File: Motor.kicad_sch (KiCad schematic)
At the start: 5 parts, among them U8 DRV8833PW

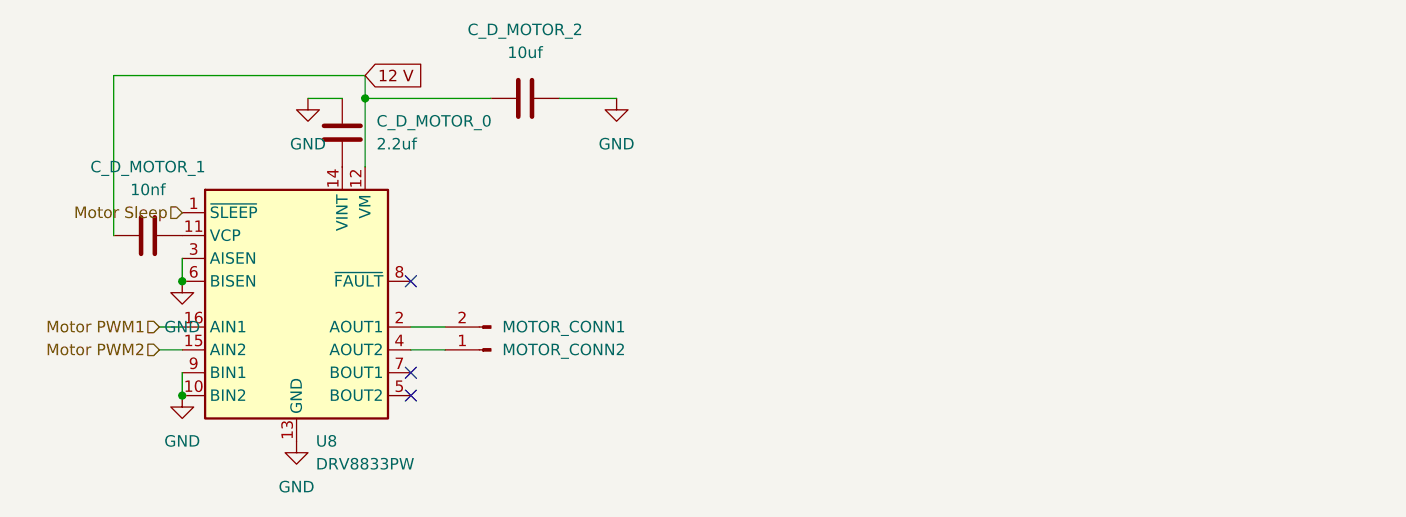
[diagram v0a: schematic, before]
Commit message: footprints
footprints
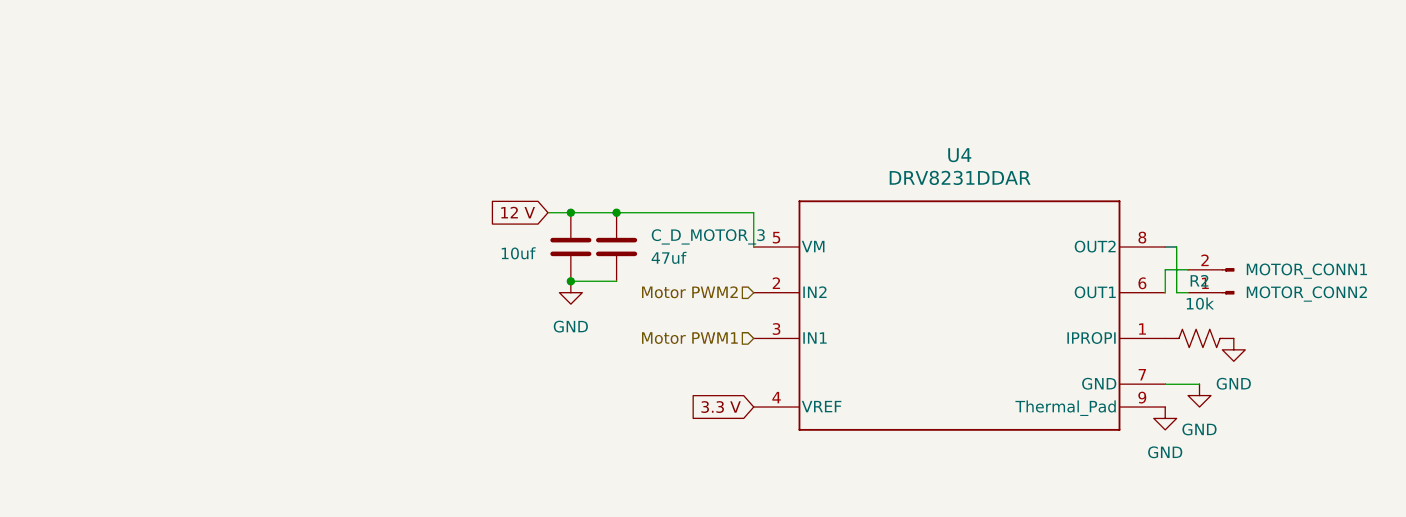
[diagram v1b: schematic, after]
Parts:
- removed C_D_MOTOR_0: 2.2uf, symbol Device:C
- removed C_D_MOTOR_1: 10nf, symbol Device:C
- removed U8: DRV8833PW, Package_SO:TSSOP-16_4.4x5mm_P0.65mm, symbol Driver_Motor:DRV8833PW
- added C_D_MOTOR_3: 47uf, Capacitor_SMD:C_1206_3216Metric_Pad1.33x1.80mm_HandSolder, symbol Device:C
- added R2: 10k, symbol Device:R_US
- added U4: DRV8231DDAR, CustomFootprints:DDA0008J-IPC_A, symbol drv:DRV8231DDAR
- C_D_MOTOR_2: footprint (none) -> Capacitor_SMD:C_0603_1608Metric_Pad1.08x0.95mm_HandSolder
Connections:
- net 12 V: now also C_D_MOTOR_2.2, C_D_MOTOR_3.1, U4.5 (VM); no longer C_D_MOTOR_2.1
- net GND: now also C_D_MOTOR_2.1, C_D_MOTOR_3.2, R2.1, U4.7 (GND), U4.9 (Thermal_Pad); no longer C_D_MOTOR_2.2
- net Motor PWM1: now also U4.3 (IN1)
- net Motor PWM2: now also U4.2 (IN2)
- net at MOTOR_CONN1.2 (Pin_2): now also U4.6 (OUT1)
- net at MOTOR_CONN1.1 (Pin_1): now also U4.8 (OUT2)
- new net: R2.2, U4.1 (IPROPI)
- new net 3.3 V: U4.4 (VREF)
- no-connect marks 3 -> 0
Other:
- moved on the sheet: MOTOR_CONN1

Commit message: Finished footprints
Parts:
- R2: footprint (none) -> Capacitor_SMD:C_0603_1608Metric_Pad1.08x0.95mm_HandSolder
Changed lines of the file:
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@@
 			)
 		)
-		(property "Footprint" ""
+		(property "Footprint" "Capacitor_SMD:C_0603_1608Metric_Pad1.08x0.95mm_HandSolder"
 			(at 182.626 44.196 90)
 			(hide yes)
